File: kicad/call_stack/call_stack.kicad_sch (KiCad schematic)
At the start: 23 parts

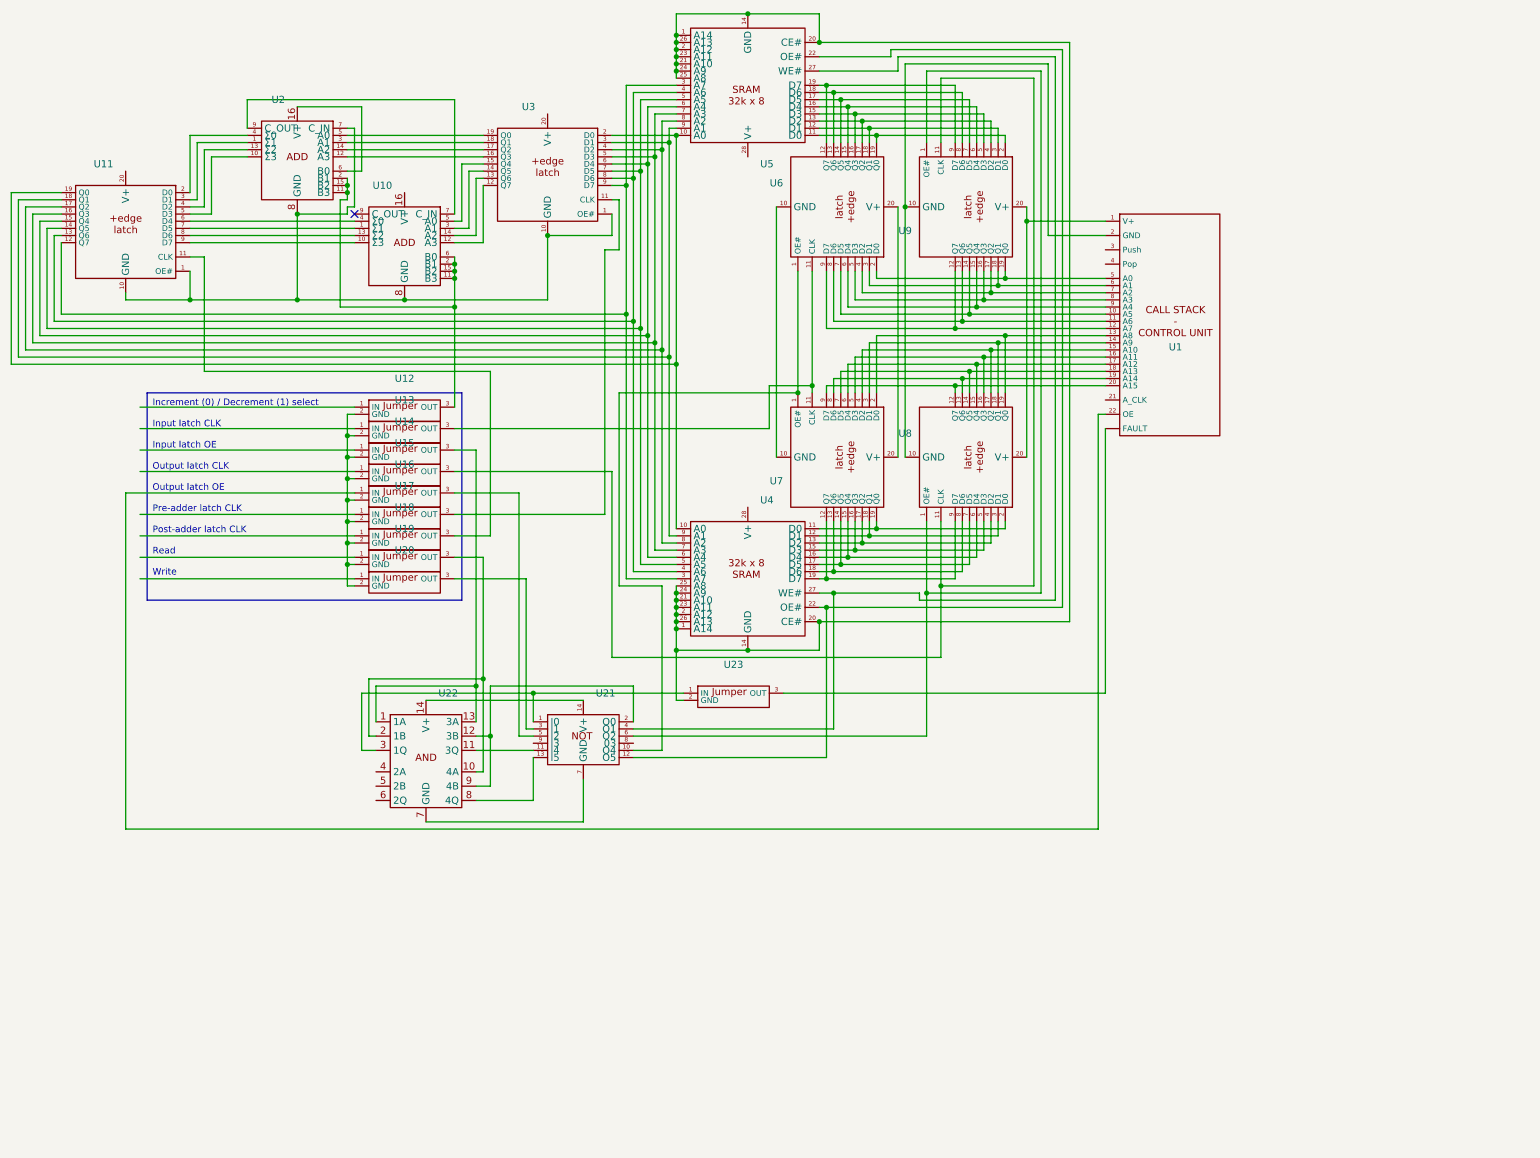
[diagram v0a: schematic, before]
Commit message: Completed design for call stack
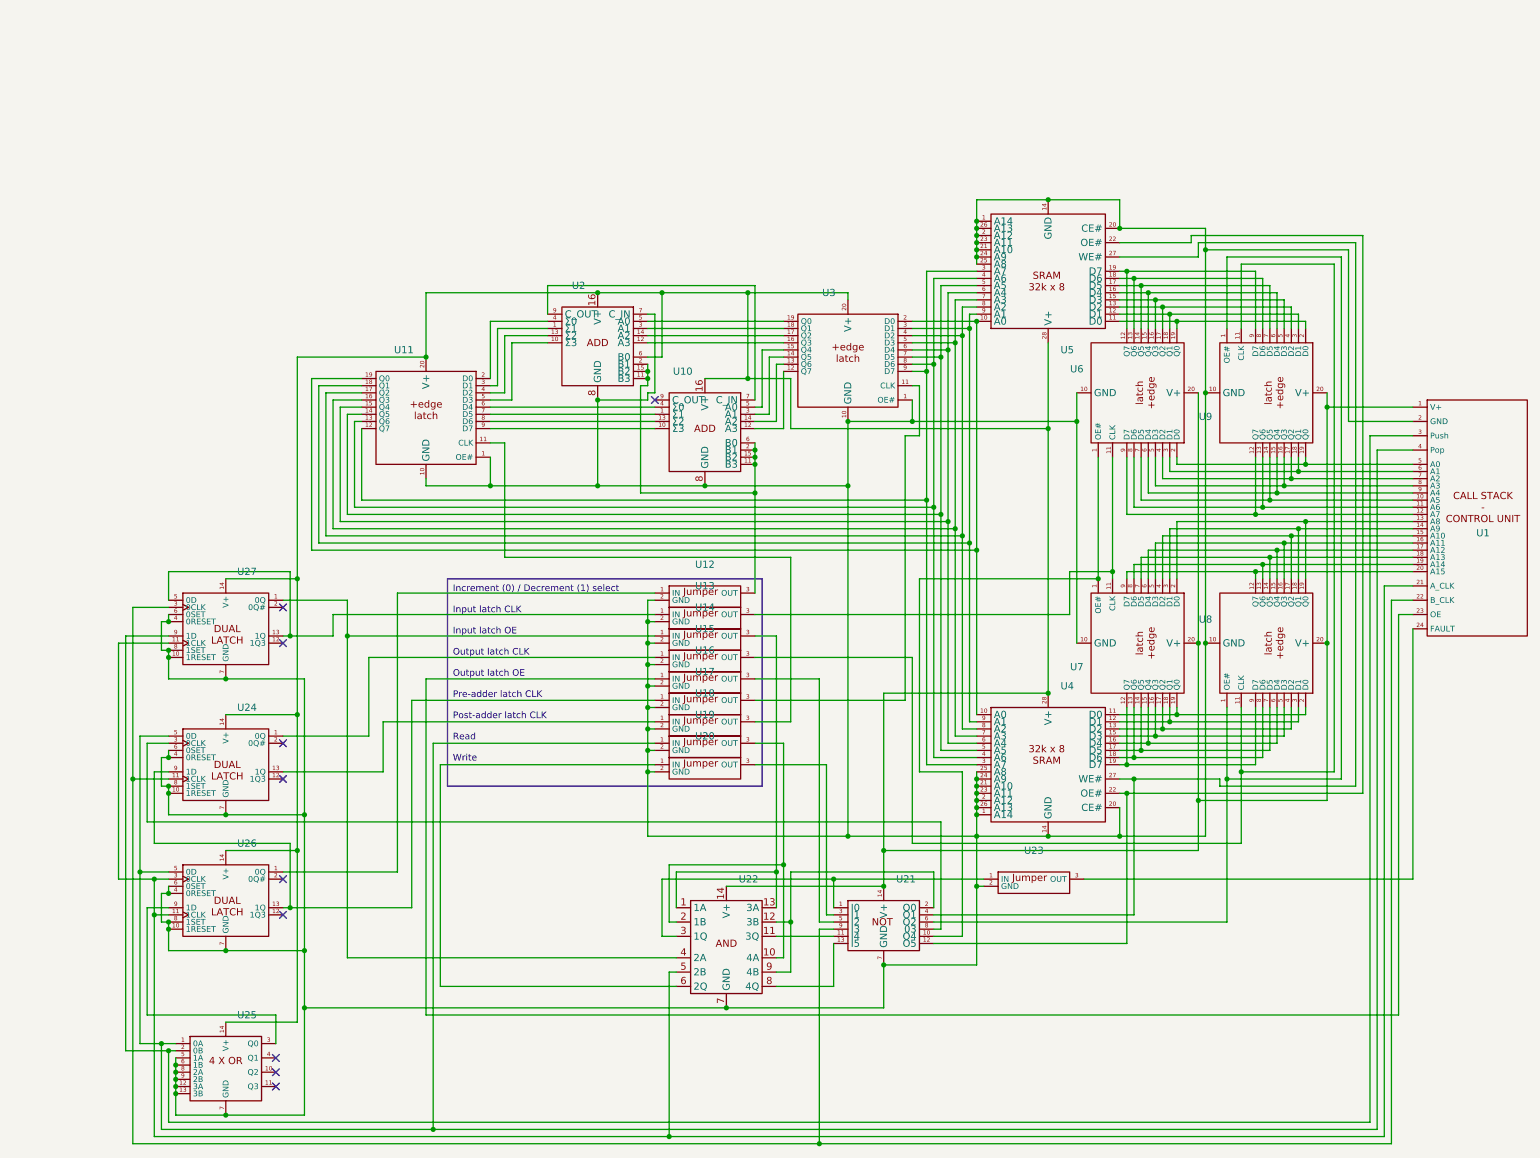
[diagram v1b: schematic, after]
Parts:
- added U24, U26, U27: ~, Package_DIP:DIP-14_W7.62mm, symbol custom_symbol_lib:dual_latch
- added U25: ~, Package_DIP:DIP-14_W7.62mm, symbol custom_symbol_lib:quad_OR
- U1: footprint Connector_PinHeader_2.54mm:PinHeader_1x23_P2.54mm_Vertical -> Connector_PinHeader_2.54mm:PinHeader_1x24_P2.54mm_Vertical
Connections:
- net at U23.3 (OUT): now also U1.24 (FAULT); no longer U1. (FAULT)
- net at U1.1 (V+), U8.20 (V+), U9.20 (V+): now also U10.16 (V+), U11.20 (V+), U2.16 (V+), U2.6 (B0), U21.14 (V+), U22.14 (V+), U3.20 (V+), U4.28 (V+), U5.28 (V+), U6.20 (V+), U7.20 (V+), U24.14 (V+), U25.14 (V+), U26.14 (V+), U27.14 (V+)
- net at U1.2 (GND), U8.10 (GND), U9.10 (GND): now also U10.8 (GND), U11.1 (OE#), U11.10 (GND), U12.2 (GND), U13.2 (GND), U14.2 (GND), U15.2 (GND), U16.2 (GND), U17.2 (GND), U18.2 (GND), U19.2 (GND), U2.7 (C_IN), U2.8 (GND), U20.2 (GND), U21.7 (GND), U22.7 (GND), U23.2 (GND), U3.1 (OE#), U3.10 (GND), U4.1 (A14), U4.14 (GND), U4.2 (A12), U4.20 (CE#), U4.21 (A10), U4.23 (A11), U4.24 (A9), U4.25 (A8), U4.26 (A13), U5.1 (A14), U5.14 (GND), U5.2 (A12), U5.20 (CE#), U5.21 (A10), U5.23 (A11), U5.24 (A9), U5.25 (A8), U5.26 (A13), U6.10 (GND), U7.10 (GND), U24.10 (1RESET), U24.4 (0RESET), U24.6 (0SET), U24.7 (GND), U24.8 (1SET), U25.12 (3A), U25.13 (3B), U25.5 (1A), U25.6 (1B), U25.7 (GND), U25.8 (2A), U25.9 (2B), U26.10 (1RESET), U26.4 (0RESET), U26.6 (0SET), U26.7 (GND), U26.8 (1SET), U27.10 (1RESET), U27.4 (0RESET), U27.6 (0SET), U27.7 (GND), U27.8 (1SET)
- net at U1.21 (A_CLK): now also U22.5 (2B), U26.11 (1CLK), U26.3 (0CLK), U27.11 (1CLK)
- net at U1.22 (B_CLK): now also U21.9 (I3), U24.11 (1CLK), U27.3 (0CLK); no longer U16.1 (IN)
- net at U1.3 (Push): now also U25.2 (0B), U27.9 (1D)
- net at U1.4 (Pop): now also U19.1 (IN), U24.5 (0D), U25.1 (0A), U26.5 (0D)
- net at U14.1 (IN): now also U22.4 (2A), U27.1 (0Q)
- net at U20.1 (IN): now also U22.6 (2Q)
- net at U15.1 (IN): now also U24.1 (0Q)
- net at U18.1 (IN): now also U24.13 (1Q)
- net at U21.8 (03): now also U24.3 (0CLK)
- net at U12.1 (IN): now also U26.1 (0Q)
- net at U13.1 (IN): now also U27.13 (1Q), U27.5 (0D)
- net at U17.1 (IN): now also U24.9 (1D), U26.13 (1Q)
- new net: U1.23 (OE), U16.1 (IN)
- new net: U25.3 (Q0), U26.9 (1D)
- no-connect marks 1 -> 10
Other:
- moved on the sheet: U10, U11, U12, U13, U14, U15, U16, U17, U18, U19, U2, U20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

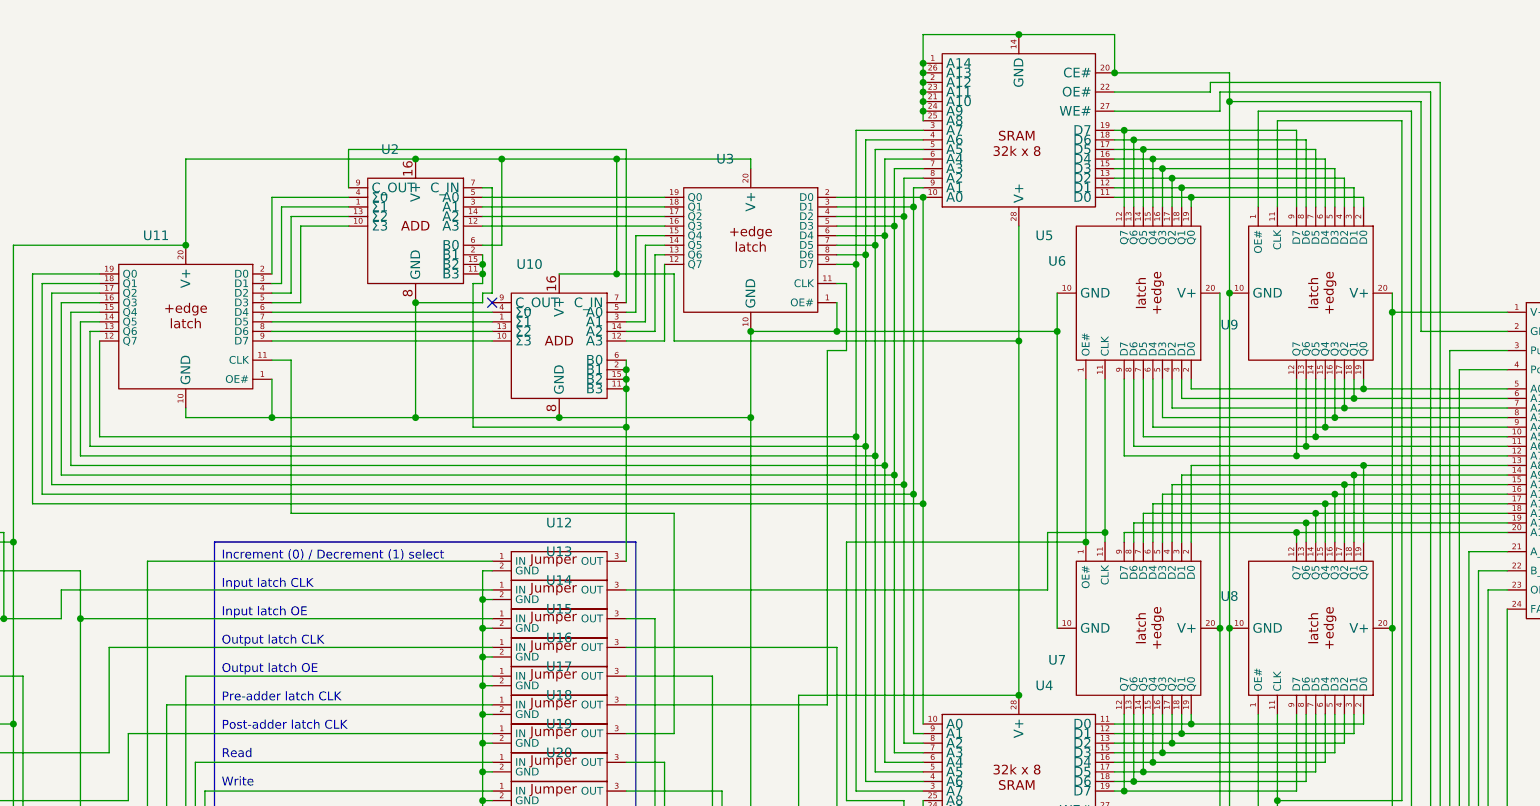
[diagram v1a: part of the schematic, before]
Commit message: stuff
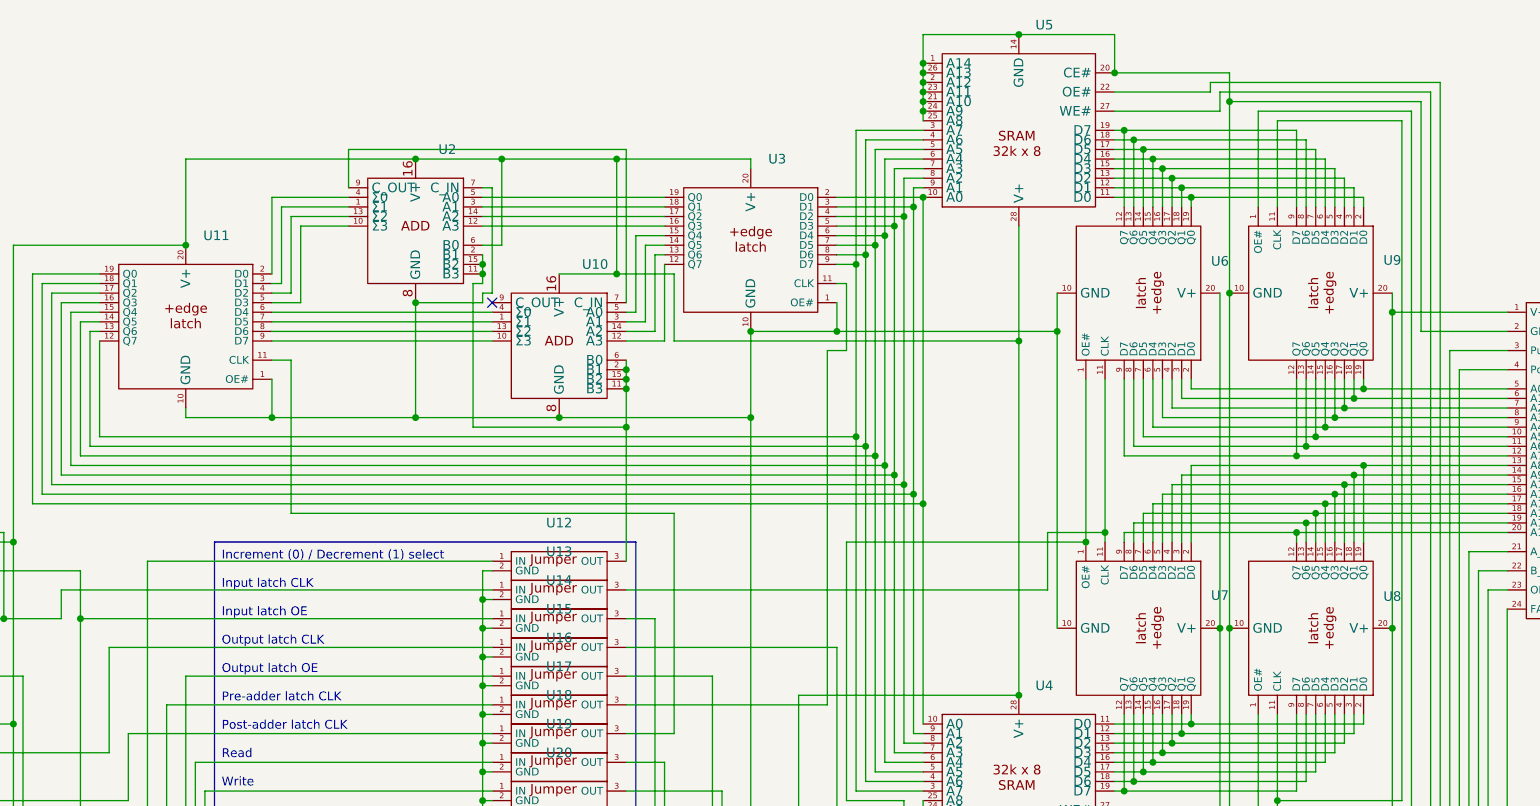
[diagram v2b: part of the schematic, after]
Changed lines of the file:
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@@
 		)
 		(property "Footprint" "Connector_PinHeader_2.54mm:PinHeader_1x24_P2.54mm_Vertical"
-			(at 329.184 123.444 0)
+			(at 329.184 125.73 0)
 			(effects
 				(font
@@
 		(fields_autoplaced yes)
 		(property "Reference" "U11"
-			(at 140.0459 73.66 0)
-			(effects
-				(font
-					(size 1.27 1.27)
-				)
-				(justify left)
-			)
-		)
-		(property "Value" "~"
-			(at 140.0459 76.2 0)
-			(effects
-				(font
-					(size 1.27 1.27)
-				)
-				(justify left)
+			(at 144.5581 73.66 0)
+			(effects
+				(font
+					(size 1.27 1.27)
+				)
+				(justify right)
+			)
+		)
+		(property "Value" "~"
+			(at 144.5581 76.2 0)
+			(effects
+				(font
+					(size 1.27 1.27)
+				)
+				(justify right)
 			)
 		)
@@
 		(fields_autoplaced yes)
 		(property "Reference" "U7"
-			(at 257.81 129.9562 90)
-			(effects
-				(font
-					(size 1.27 1.27)
-				)
-			)
-		)
-		(property "Value" "~"
-			(at 257.81 128.0511 90)
+			(at 279.4 121.3798 90)
+			(effects
+				(font
+					(size 1.27 1.27)
+				)
+			)
+		)
+		(property "Value" "~"
+			(at 279.4 123.2849 90)
 			(effects
 				(font
@@
 		(fields_autoplaced yes)
 		(property "Reference" "U2"
-			(at 170.5259 62.23 0)
-			(effects
-				(font
-					(size 1.27 1.27)
-				)
-				(justify left)
-			)
-		)
-		(property "Value" "~"
-			(at 170.5259 64.77 0)
-			(effects
-				(font
-					(size 1.27 1.27)
-				)
-				(justify left)
+			(at 175.7365 62.23 0)
+			(effects
+				(font
+					(size 1.27 1.27)
+				)
+				(justify right)
+			)
+		)
+		(property "Value" "~"
+			(at 175.7365 64.77 0)
+			(effects
+				(font
+					(size 1.27 1.27)
+				)
+				(justify right)
 			)
 		)
@@
 		(fields_autoplaced yes)
 		(property "Reference" "U3"
-			(at 214.9759 63.5 0)
-			(effects
-				(font
-					(size 1.27 1.27)
-				)
-				(justify left)
-			)
-		)
-		(property "Value" "~"
-			(at 214.9759 66.04 0)
-			(effects
-				(font
-					(size 1.27 1.27)
-				)
-				(justify left)
+			(at 219.4881 63.5 0)
+			(effects
+				(font
+					(size 1.27 1.27)
+				)
+				(justify right)
+			)
+		)
+		(property "Value" "~"
+			(at 219.4881 66.04 0)
+			(effects
+				(font
+					(size 1.27 1.27)
+				)
+				(justify right)
 			)
 		)
@@
 		(fields_autoplaced yes)
 		(property "Reference" "U5"
-			(at 254.9241 73.66 0)
+			(at 254.9241 45.72 0)
 			(effects
 				(font
@@
 		)
 		(property "Value" "~"
-			(at 254.9241 71.12 0)
+			(at 254.9241 48.26 0)
 			(effects
 				(font
@@
 		(fields_autoplaced yes)
 		(property "Reference" "U8"
-			(at 280.67 121.5038 90)
-			(effects
-				(font
-					(size 1.27 1.27)
-				)
-			)
-		)
-		(property "Value" "~"
-			(at 280.67 123.4089 90)
+			(at 302.26 121.5038 90)
+			(effects
+				(font
+					(size 1.27 1.27)
+				)
+			)
+		)
+		(property "Value" "~"
+			(at 302.26 123.4089 90)
 			(effects
 				(font
@@
 		(fields_autoplaced yes)
 		(property "Reference" "U10"
-			(at 189.5759 77.47 0)
-			(effects
-				(font
-					(size 1.27 1.27)
-				)
-				(justify left)
-			)
-		)
-		(property "Value" "~"
-			(at 189.5759 80.01 0)
-			(effects
-				(font
-					(size 1.27 1.27)
-				)
-				(justify left)
+			(at 194.7865 77.47 0)
+			(effects
+				(font
+					(size 1.27 1.27)
+				)
+				(justify right)
+			)
+		)
+		(property "Value" "~"
+			(at 194.7865 80.01 0)
+			(effects
+				(font
+					(size 1.27 1.27)
+				)
+				(justify right)
 			)
 		)
@@
 		(fields_autoplaced yes)
 		(property "Reference" "U9"
-			(at 280.67 85.5062 90)
-			(effects
-				(font
-					(size 1.27 1.27)
-				)
-			)
-		)
-		(property "Value" "~"
-			(at 280.67 83.6011 90)
+			(at 302.26 76.9298 90)
+			(effects
+				(font
+					(size 1.27 1.27)
+				)
+			)
+		)
+		(property "Value" "~"
+			(at 302.26 78.8349 90)
 			(effects
 				(font
@@
 		(fields_autoplaced yes)
 		(property "Reference" "U6"
-			(at 257.81 77.0538 90)
-			(effects
-				(font
-					(size 1.27 1.27)
-				)
-			)
-		)
-		(property "Value" "~"
-			(at 257.81 78.9589 90)
-			(effects
-				(font
+			(at 279.4 77.0538 90)
+			(effects
+				(font
+					(size 1.27 1.27)
+				)
+			)
+		)
+		(property "Value" "~"
+			(at 279.4 78.9589 90)
+			(effects
+				(font
